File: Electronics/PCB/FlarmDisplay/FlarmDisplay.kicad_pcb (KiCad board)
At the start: 2 copper layers, 43 x 25 mm, 65 parts, among them J1 RJ12, J2 SWD, SW1 RESET, SW2 BOOT, U1 IPN80R3K3P7ATMA1, U2 STM32F334K8Ux, U3 TLC5928, U4 TLC5928, Y1 16MHz

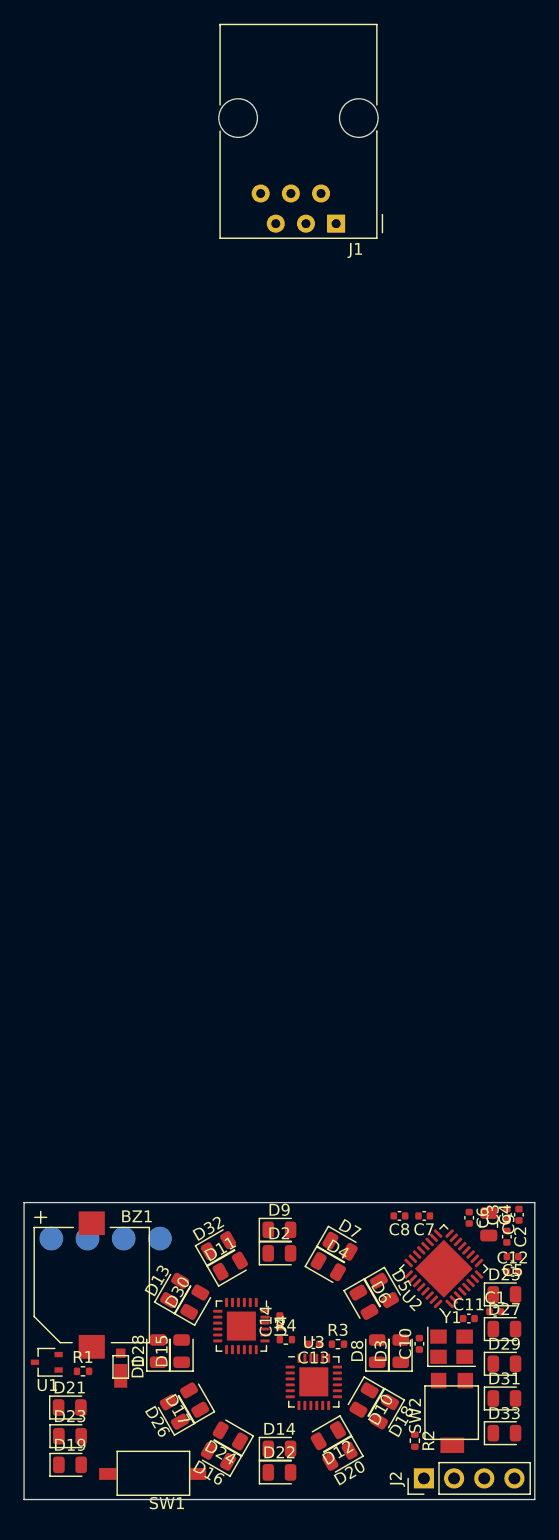
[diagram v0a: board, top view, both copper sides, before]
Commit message: Latest
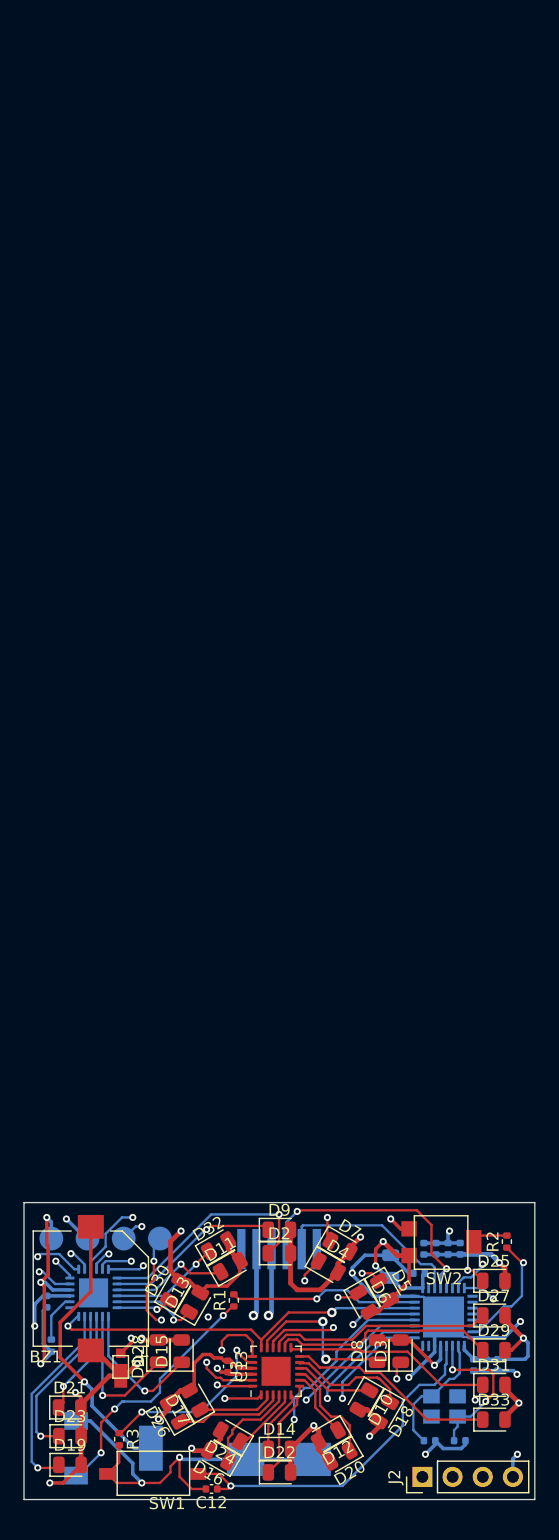
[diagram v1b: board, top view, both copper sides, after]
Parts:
- C1, C10, C11, C14, C2, C3, C4, C5, C6, C7, C8, C9, R4, U2, U4, Y1: moved to B.Cu
- J1: footprint Connector_RJ:RJ12_Amphenol_54601 -> FlarmDisplay:RJE231660413T; moved to B.Cu
- U1: footprint Package_TO_SOT_SMD:SOT-323_SC-70 -> Package_TO_SOT_SMD:SOT-223-3_TabPin2; moved to B.Cu
- moved J1 95.1 mm to (101.5, 122.5), turned to 270 degrees
- moved C12 31.3 mm to (95.8, 134.1), turned to 180 degrees
- moved R3 20.1 mm to (88.0, 129.9), turned to 270 degrees
- moved R4 19.8 mm to (82.3, 122.0), turned to 270 degrees
- moved C14 19.7 mm to (81.9, 118.3), turned to 270 degrees
- moved R2 18.5 mm to (120.7, 113.3), turned to 90 degrees
- moved SW2 14.3 mm to (115.1, 113.4), turned to 90 degrees
- moved R1 14.0 mm to (97.7, 118.2), turned to 90 degrees
- moved C7 14.0 mm to (119.9, 123.7), turned to 270 degrees
- moved U4 12.8 mm to (85.9, 117.6)
- moved C6 12.5 mm to (118.9, 123.7)
- moved C11 10.3 mm to (116.7, 130.0)
- moved U1 9.16 mm to (87.5, 130.7), turned to 0 degrees
- moved C9 8.99 mm to (110.9, 115.4), turned to 90 degrees
- moved C10 8.20 mm to (114.1, 130.0), turned to 0 degrees
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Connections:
- net ERR_READ renamed Net-(U4-Pad19)
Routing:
- net +3V3: track 0.00 -> 161.2 mm, vias 0 -> 19
- net GND: track 0.00 -> 128.0 mm, vias 0 -> 15
- net Net-(U2-Pad13): track 0.00 -> 50.0 mm, vias 0 -> 3
- net Net-(U2-Pad12): track 0.00 -> 46.6 mm, vias 0 -> 3
- net Net-(TP3-Pad1): track 0.00 -> 35.8 mm, vias 0 -> 3
- net Net-(D3-Pad1): track 0.00 -> 35.3 mm, vias 0 -> 2
- net Net-(TP4-Pad1): track 0.00 -> 35.0 mm, vias 0 -> 3
- net Net-(U2-Pad14): track 0.00 -> 32.7 mm, vias 0 -> 2
- net Net-(BZ1-Pad2): track 0.00 -> 30.8 mm, vias 0 -> 2
- net NRST: track 0.00 -> 30.0 mm, vias 0 -> 1
- net Net-(D6-Pad1): track 0.00 -> 28.3 mm, vias 0 -> 2
- net Net-(D5-Pad1): track 0.00 -> 26.7 mm, vias 0 -> 2
- net Net-(U2-Pad11): track 0.00 -> 26.3 mm, vias 0 -> 2
- net Net-(U3-Pad19): track 0.00 -> 26.1 mm, vias 0 -> 2
- net SWDAT: track 0.00 -> 25.2 mm, vias 0 -> 2
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- added copper zone on In1.Cu, net +3V3
- added copper zone on In2.Cu, net GND
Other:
- copper layers 2 -> 4
